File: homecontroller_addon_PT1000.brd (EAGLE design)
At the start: 60 x 100 mm, 48 parts, among them U1 OPA2188AIDGKR, U2 OPA2188AIDGKR, U3 REF3025AIDBZTG4, U4 ADS1015IDGST, X1 S2L3.50/10/90G

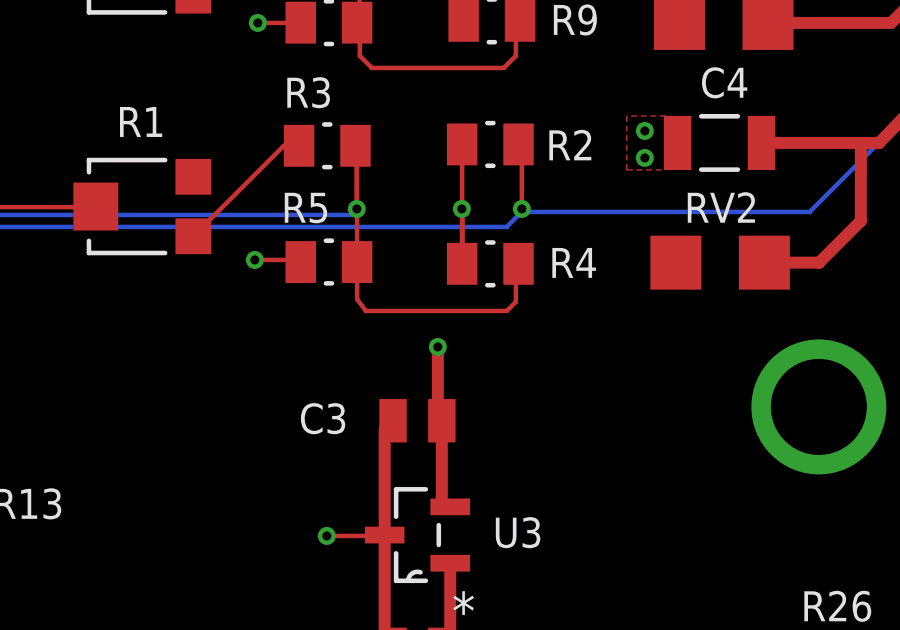
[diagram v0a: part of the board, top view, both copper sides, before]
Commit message: update
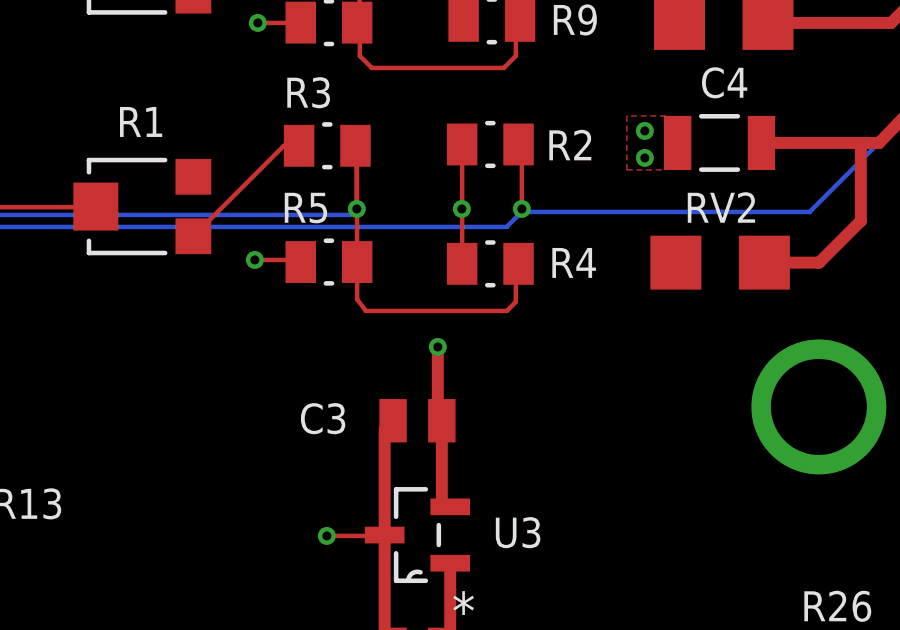
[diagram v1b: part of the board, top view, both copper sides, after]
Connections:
- new net REF2.5V: C3.2, R2.1, R4.2, U3.2
- net REF2.0V: no longer C3.2, R2.1, R4.2, U3.2
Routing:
- net REF2.0V: track 58.3 -> 49.4 mm
- net REF2.5V: track 0.00 -> 6.97 mm
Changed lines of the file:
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@@
 </signal>
 <signal name="REF2.0V">
-<contactref element="U3" pad="2"/>
-<contactref element="R2" pad="1"/>
-<contactref element="R4" pad="2"/>
-<contactref element="C3" pad="2"/>
 <contactref element="R9" pad="2"/>
 <contactref element="R10" pad="1"/>
@@
 <wire x1="33.5" y1="82.9" x2="31.9" y2="82.9" width="1" layer="15"/>
 <via x="33.4" y="66.8" extent="1-16" drill="0.3"/>
-<wire x1="33.4102" y1="64.97" x2="33.4102" y2="68.95" width="0.15" layer="1"/>
-<wire x1="32.7328" y1="59.74" x2="32.7328" y2="57.1492" width="0.4" layer="1"/>
-<wire x1="32.7328" y1="57.1492" x2="33.0122" y2="56.8698" width="0.15" layer="1"/>
 <via x="32.6" y="62.2" extent="1-16" drill="0.3"/>
 <wire x1="32.6" y1="62.2" x2="32.6" y2="59.8728" width="0.4" layer="1"/>
-<wire x1="32.6" y1="59.8728" x2="32.7328" y2="59.74" width="0.15" layer="1"/>
-<wire x1="33.4102" y1="64.97" x2="33.4102" y2="66.7898" width="0.15" layer="1"/>
 <wire x1="33.4102" y1="66.7898" x2="33.4" y2="66.8" width="0.15" layer="1"/>
 <wire x1="33.4" y1="66.8" x2="31.9" y2="66.8" width="1" layer="15"/>
@@
 </polygon>
 </signal>
+<signal name="REF2.5V">
+<contactref element="U3" pad="2"/>
+<contactref element="R2" pad="1"/>
+<contactref element="R4" pad="2"/>
+<contactref element="C3" pad="2"/>
+<wire x1="33.4102" y1="64.97" x2="33.4102" y2="68.95" width="0.15" layer="1"/>
+<wire x1="32.7328" y1="59.74" x2="32.7328" y2="57.1492" width="0.4" layer="1"/>
+<wire x1="32.7328" y1="57.1492" x2="33.0122" y2="56.8698" width="0.15" layer="1"/>
+<wire x1="32.7328" y1="59.74" x2="33.4102" y2="64.97" width="0" layer="19" extent="1-1"/>
+</signal>
 </signals>
